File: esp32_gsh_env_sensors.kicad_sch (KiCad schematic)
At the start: 54 parts, among them J1 USB_C_Receptacle_USB2.0, J2 C50950, J4 C2718488, Q1 SS8050, Q2 SS8050, SW1 EN, SW2 BOOT, SW3 CALIBRATE, U1 MP2359, U2 BME280, U3 CH340G, U4 MH-Z19B, U5 ESP32-WROOM-32E, Y1 12MHz

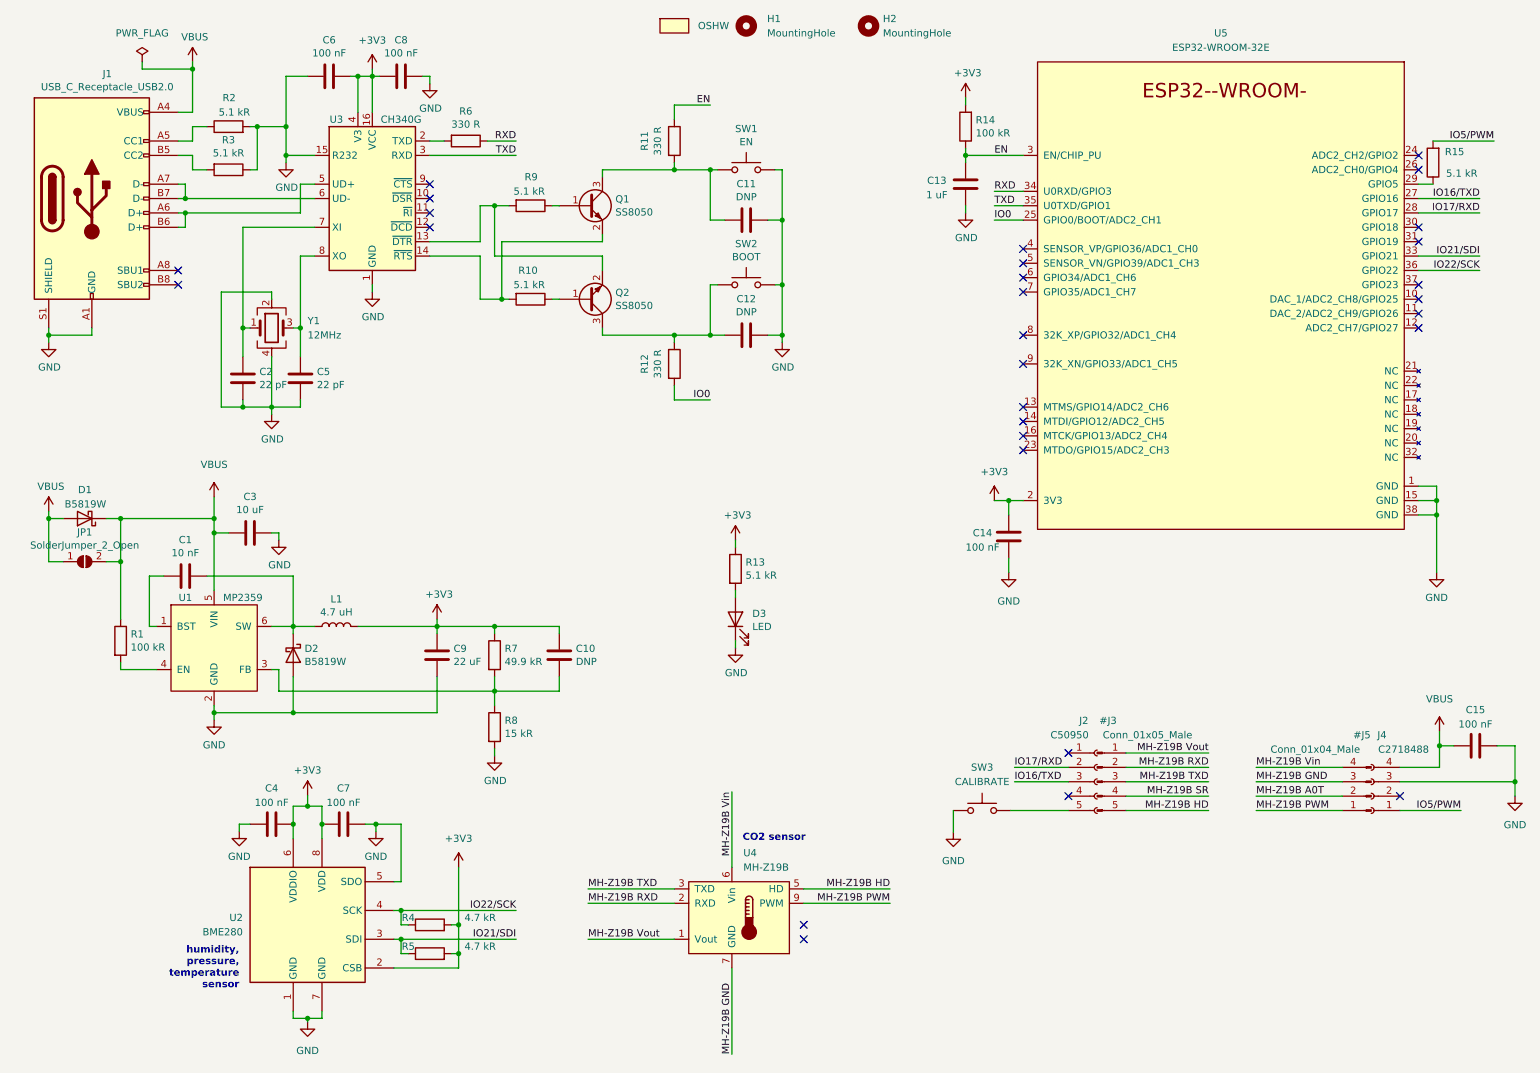
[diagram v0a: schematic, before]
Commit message: Update schematics
- Rename existing mounting holes to tooling holes
- Add mounting holes
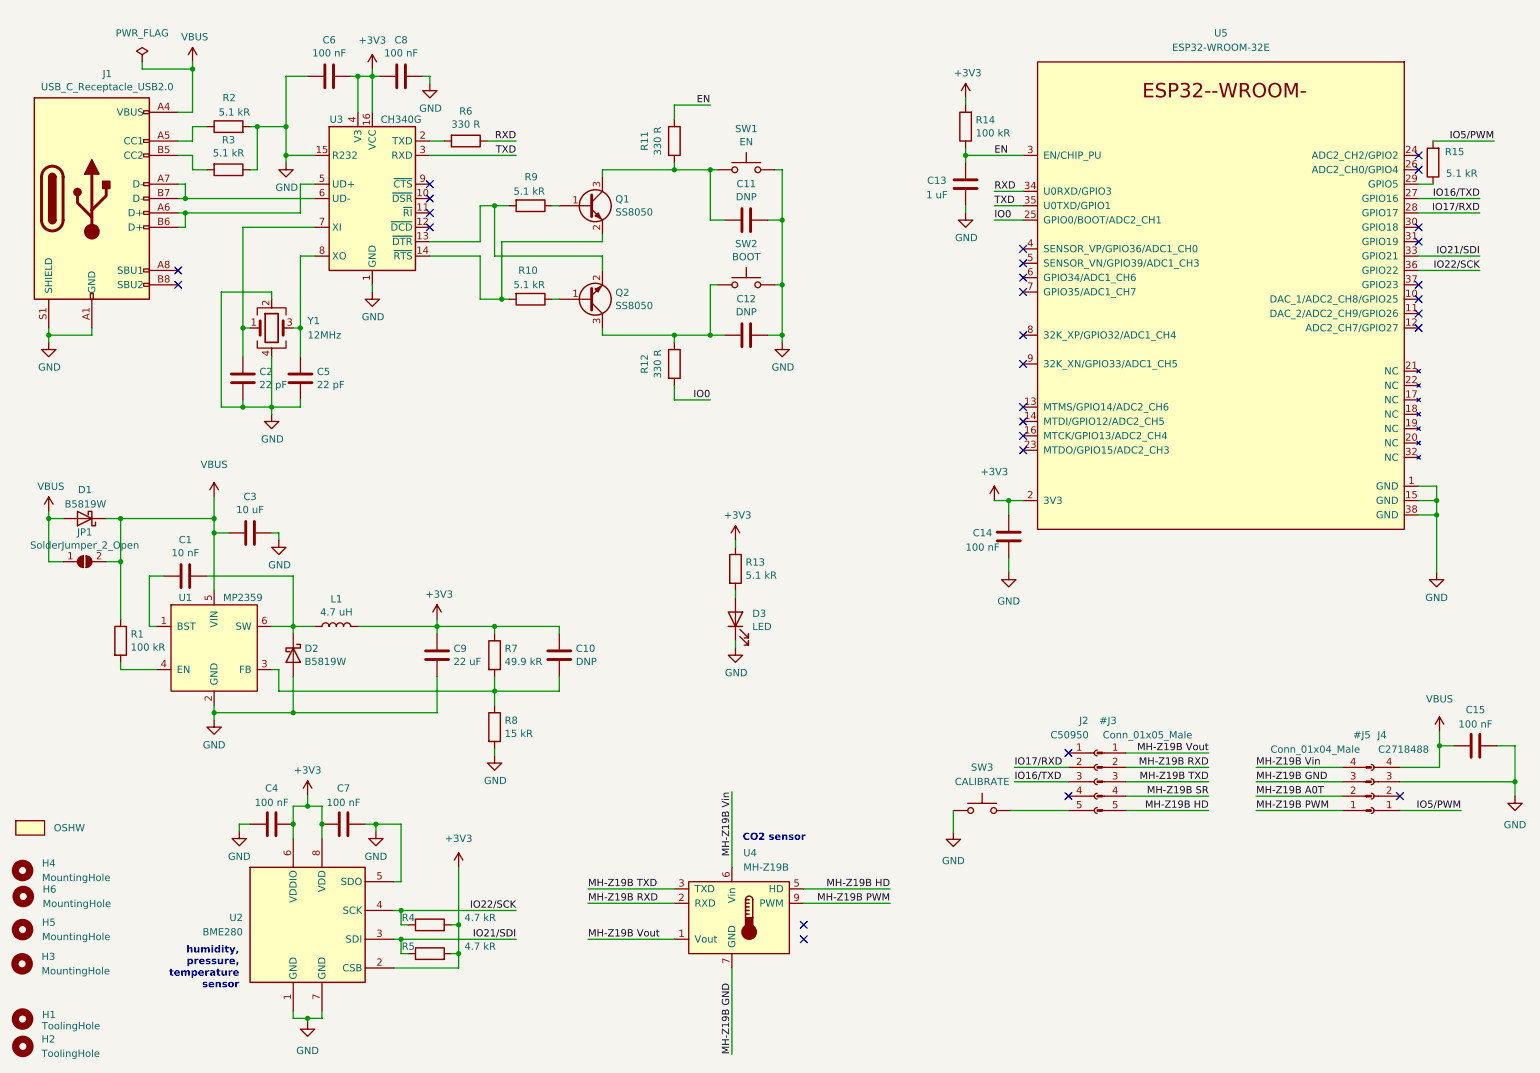
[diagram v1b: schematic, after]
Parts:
- added H3, H4, H5, H6: MountingHole, MountingHole:MountingHole_4.3mm_M4_DIN965, symbol Mechanical:MountingHole
- H1, H2: value MountingHole -> ToolingHole
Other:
- moved on the sheet: H1, H2
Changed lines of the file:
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@@
     (pin "2")
+  )
+  (symbol (lib_id "Mechanical:MountingHole") (at 14.5542 168.9862 0) (unit 1)
+    (in_bom yes) (on_board yes) (fields_autoplaced)
+    (property "Reference" "H6" (id 0) (at 17.9832 167.7161 0)
+      (effects (font (size 1.27 1.27)) (justify left))
+    )
+    (property "Value" "MountingHole" (id 1) (at 17.9832 170.2561 0)
+      (effects (font (size 1.27 1.27)) (justify left))
+    )
+    (property "Footprint" "MountingHole:MountingHole_4.3mm_M4_DIN965" (id 2) (at 14.5542 168.9862 0)
+      (effects (font (size 1.27 1.27)) hide)
+    )
+    (property "Datasheet" "~" (id 3) (at 14.5542 168.9862 0)
+      (effects (font (size 1.27 1.27)) hide)
+    )
   )
   (symbol (lib_id "Device:R") (at 129.54 74.93 0) (unit 1)
@@
     (pin "2")
   )
-  (symbol (lib_id "Mechanical:MountingHole") (at 163.83 15.24 0) (unit 1)
-    (in_bom yes) (on_board yes) (fields_autoplaced)
-    (property "Reference" "H2" (id 0) (at 166.37 13.9699 0)
-      (effects (font (size 1.27 1.27)) (justify left))
-    )
-    (property "Value" "MountingHole" (id 1) (at 166.37 16.5099 0)
-      (effects (font (size 1.27 1.27)) (justify left))
-    )
-    (property "Footprint" "ToolingHole:ToolingHole_JLCSMT" (id 2) (at 163.83 15.24 0)
-      (effects (font (size 1.27 1.27)) hide)
-    )
-    (property "Datasheet" "~" (id 3) (at 163.83 15.24 0)
+  (symbol (lib_id "Mechanical:MountingHole") (at 14.478 195.453 0) (unit 1)
+    (in_bom yes) (on_board yes) (fields_autoplaced)
+    (property "Reference" "H2" (id 0) (at 17.78 194.1829 0)
+      (effects (font (size 1.27 1.27)) (justify left))
+    )
+    (property "Value" "ToolingHole" (id 1) (at 17.78 196.7229 0)
+      (effects (font (size 1.27 1.27)) (justify left))
+    )
+    (property "Footprint" "ToolingHole:ToolingHole_JLCSMT" (id 2) (at 14.478 195.453 0)
+      (effects (font (size 1.27 1.27)) hide)
+    )
+    (property "Datasheet" "~" (id 3) (at 14.478 195.453 0)
       (effects (font (size 1.27 1.27)) hide)
     )
@@
     (pin "1")
   )
-  (symbol (lib_id "Mechanical:MountingHole") (at 142.24 15.24 0) (unit 1)
-    (in_bom yes) (on_board yes) (fields_autoplaced)
-    (property "Reference" "H1" (id 0) (at 145.923 13.9699 0)
-      (effects (font (size 1.27 1.27)) (justify left))
-    )
-    (property "Value" "MountingHole" (id 1) (at 145.923 16.5099 0)
-      (effects (font (size 1.27 1.27)) (justify left))
-    )
-    (property "Footprint" "ToolingHole:ToolingHole_JLCSMT" (id 2) (at 142.24 15.24 0)
-      (effects (font (size 1.27 1.27)) hide)
-    )
-    (property "Datasheet" "~" (id 3) (at 142.24 15.24 0)
+  (symbol (lib_id "Mechanical:MountingHole") (at 14.4272 190.627 0) (unit 1)
+    (in_bom yes) (on_board yes)
+    (property "Reference" "H1" (id 0) (at 17.8816 189.865 0)
+      (effects (font (size 1.27 1.27)) (justify left))
+    )
+    (property "Value" "ToolingHole" (id 1) (at 17.8308 191.8462 0)
+      (effects (font (size 1.27 1.27)) (justify left))
+    )
+    (property "Footprint" "ToolingHole:ToolingHole_JLCSMT" (id 2) (at 14.4272 190.627 0)
+      (effects (font (size 1.27 1.27)) hide)
+    )
+    (property "Datasheet" "~" (id 3) (at 14.4272 190.627 0)
+      (effects (font (size 1.27 1.27)) hide)
+    )
+  )
+  (symbol (lib_id "Mechanical:MountingHole") (at 14.4272 164.3888 0) (unit 1)
+    (in_bom yes) (on_board yes) (fields_autoplaced)
+    (property "Reference" "H4" (id 0) (at 17.8562 163.1187 0)
+      (effects (font (size 1.27 1.27)) (justify left))
+    )
+    (property "Value" "MountingHole" (id 1) (at 17.8562 165.6587 0)
+      (effects (font (size 1.27 1.27)) (justify left))
+    )
+    (property "Footprint" "MountingHole:MountingHole_4.3mm_M4_DIN965" (id 2) (at 14.4272 164.3888 0)
+      (effects (font (size 1.27 1.27)) hide)
+    )
+    (property "Datasheet" "~" (id 3) (at 14.4272 164.3888 0)
       (effects (font (size 1.27 1.27)) hide)
     )
@@
     (pin "1")
   )
+  (symbol (lib_id "Mechanical:MountingHole") (at 14.351 180.8734 0) (unit 1)
+    (in_bom yes) (on_board yes) (fields_autoplaced)
+    (property "Reference" "H3" (id 0) (at 17.78 179.6033 0)
+      (effects (font (size 1.27 1.27)) (justify left))
+    )
+    (property "Value" "MountingHole" (id 1) (at 17.78 182.1433 0)
+      (effects (font (size 1.27 1.27)) (justify left))
+    )
+    (property "Footprint" "MountingHole:MountingHole_4.3mm_M4_DIN965" (id 2) (at 14.351 180.8734 0)
+      (effects (font (size 1.27 1.27)) hide)
+    )
+    (property "Datasheet" "~" (id 3) (at 14.351 180.8734 0)
+      (effects (font (size 1.27 1.27)) hide)
+    )
+  )
   (symbol (lib_id "Device:R") (at 180.975 33.02 180) (unit 1)
     (in_bom yes) (on_board yes)
@@
     (pin "1")
     (pin "2")
+  )
+  (symbol (lib_id "Mechanical:MountingHole") (at 14.4272 174.8282 0) (unit 1)
+    (in_bom yes) (on_board yes) (fields_autoplaced)
+    (property "Reference" "H5" (id 0) (at 17.8562 173.5581 0)
+      (effects (font (size 1.27 1.27)) (justify left))
+    )
+    (property "Value" "MountingHole" (id 1) (at 17.8562 176.0981 0)
+      (effects (font (size 1.27 1.27)) (justify left))
+    )
+    (property "Footprint" "MountingHole:MountingHole_4.3mm_M4_DIN965" (id 2) (at 14.4272 174.8282 0)
+      (effects (font (size 1.27 1.27)) hide)
+    )
+    (property "Datasheet" "~" (id 3) (at 14.4272 174.8282 0)
+      (effects (font (size 1.27 1.27)) hide)
+    )
   )
   (symbol (lib_id "Device:R") (at 129.54 35.56 0) (unit 1)
@@
     (pin "1")
   )
-  (symbol (lib_id "Icon:Icon") (at 129.54 15.2146 0) (unit 1)
-    (in_bom yes) (on_board yes) (fields_autoplaced)
-    (property "Reference" "I1" (id 0) (at 129.54 15.2146 0)
-      (effects (font (size 1.27 1.27)) hide)
-    )
-    (property "Value" "OSHW" (id 1) (at 133.7056 15.2145 0)
-      (effects (font (size 1.27 1.27)) (justify left))
-    )
-    (property "Footprint" "Symbol:OSHW-Logo2_9.8x8mm_SilkScreen" (id 2) (at 129.54 15.2146 0)
-      (effects (font (size 1.27 1.27)) hide)
-    )
-    (property "Datasheet" "" (id 3) (at 129.54 15.2146 0)
+  (symbol (lib_id "Icon:Icon") (at 15.7734 156.8704 0) (unit 1)
+    (in_bom yes) (on_board yes) (fields_autoplaced)
+    (property "Reference" "I1" (id 0) (at 15.7734 156.8704 0)
+      (effects (font (size 1.27 1.27)) hide)
+    )
+    (property "Value" "OSHW" (id 1) (at 19.939 156.8703 0)
+      (effects (font (size 1.27 1.27)) (justify left))
+    )
+    (property "Footprint" "Symbol:OSHW-Logo2_9.8x8mm_SilkScreen" (id 2) (at 15.7734 156.8704 0)
+      (effects (font (size 1.27 1.27)) hide)
+    )
+    (property "Datasheet" "" (id 3) (at 15.7734 156.8704 0)
       (effects (font (size 1.27 1.27)) hide)
     )
@@
     )
     (path "/389a456e-233e-44fa-b748-df37a931fcce"
-      (reference "H1") (unit 1) (value "MountingHole") (footprint "ToolingHole:ToolingHole_JLCSMT")
+      (reference "H1") (unit 1) (value "ToolingHole") (footprint "ToolingHole:ToolingHole_JLCSMT")
     )
     (path "/283d0aaa-ff7e-4225-aeca-e15c7d76c3fa"
-      (reference "H2") (unit 1) (value "MountingHole") (footprint "ToolingHole:ToolingHole_JLCSMT")
+      (reference "H2") (unit 1) (value "ToolingHole") (footprint "ToolingHole:ToolingHole_JLCSMT")
+    )
+    (path "/50ac6c59-da8d-4a68-ae14-f6b3b7ac48e7"
+      (reference "H3") (unit 1) (value "MountingHole") (footprint "MountingHole:MountingHole_4.3mm_M4_DIN965")
+    )
+    (path "/39ad4a79-bfea-4ab4-92ca-6389a6a5b697"
+      (reference "H4") (unit 1) (value "MountingHole") (footprint "MountingHole:MountingHole_4.3mm_M4_DIN965")
+    )
+    (path "/af5c16b8-7077-483e-9980-821b14ec5c64"
+      (reference "H5") (unit 1) (value "MountingHole") (footprint "MountingHole:MountingHole_4.3mm_M4_DIN965")
+    )
+    (path "/1d0256b9-ba48-426d-8ed6-e52e7ae5d07f"
+      (reference "H6") (unit 1) (value "MountingHole") (footprint "MountingHole:MountingHole_4.3mm_M4_DIN965")
     )
     (path "/eaf420b5-c091-4bf0-a203-4dcce8864928"
